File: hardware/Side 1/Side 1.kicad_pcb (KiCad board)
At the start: 2 copper layers, 126 x 214.2 mm, 4 parts

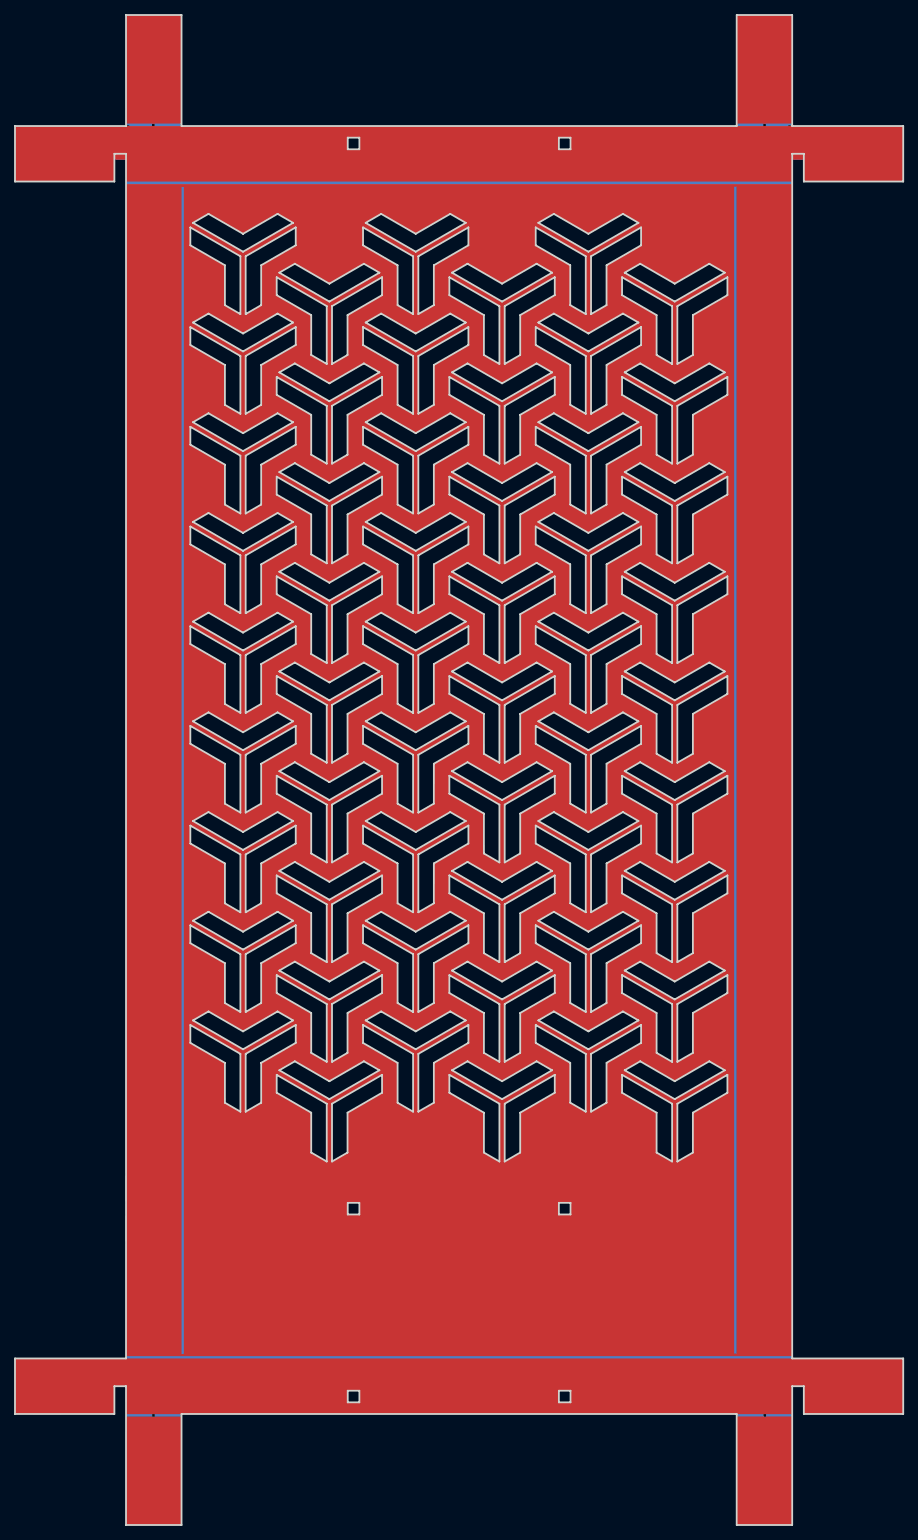
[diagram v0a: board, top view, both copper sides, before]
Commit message: God knows but a lot has changed
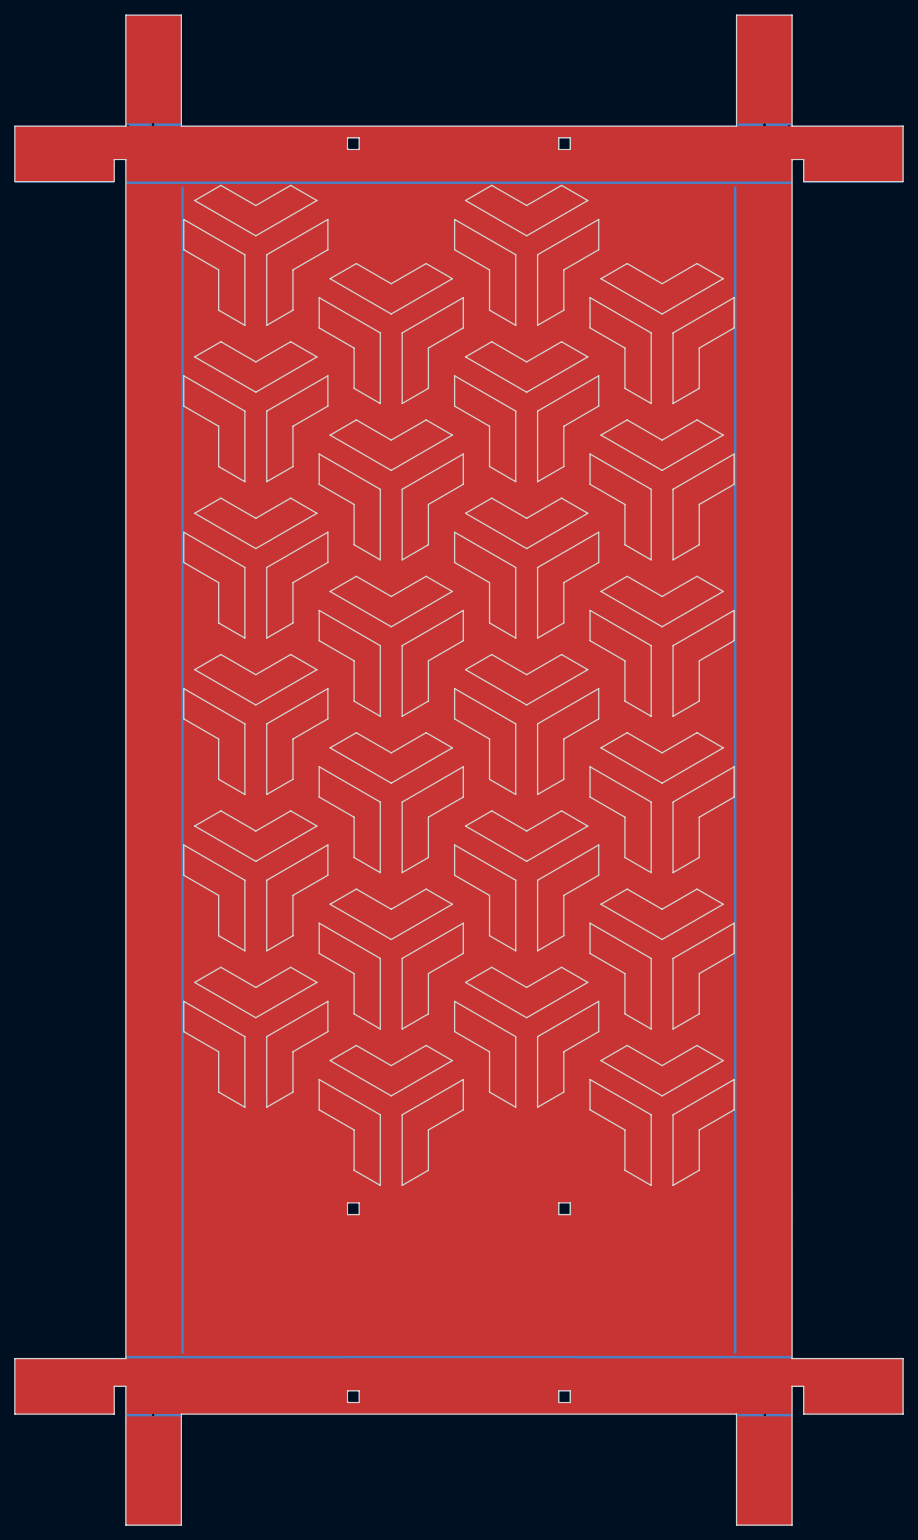
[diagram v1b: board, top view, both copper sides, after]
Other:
- outline, holes or cut-outs redrawn
- board text added: "JLCJLCJLC"
